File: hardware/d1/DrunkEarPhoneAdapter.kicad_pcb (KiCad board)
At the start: 4 copper layers, 50 x 50 mm, 188 parts, among them J3 SWD, J4 UART, Q1 CSD17577Q3A, Q2 CSD17577Q3A, Q3 DMG1012T-7, SW1 SSSS811101, SW3 DSHP02TSGER, U1 CS43131-CNZR, U10 BLM15PX601SN1D, U11 TPS7A2033PDBVR, U12 TPS7A2018PDBVR, U13 TPS7A2018PDBVR, U14 BLM15PX601SN1D, U15 ESDA25P35-1U1M, U16 ESDA25P35-1U1M, U17 SN74LVC1G32DBVR, U18 TPS22917DBVR, U19 TPS22917DBVR, U2 STM32G0B1VCT6, U20 SN74AVC4T774RSVR, U21 TCA9406DCUR, U3 TS3USB221RSER, U4 TCPP03-M20, U5 TCPP03-M20, U6 ES8327, U7 TPS7A2018PDBVR, U8 TPS7A2033PDBVR, U9 TPS560430XFDBVR, X1 22.5792MHz, X3 24.576MHz

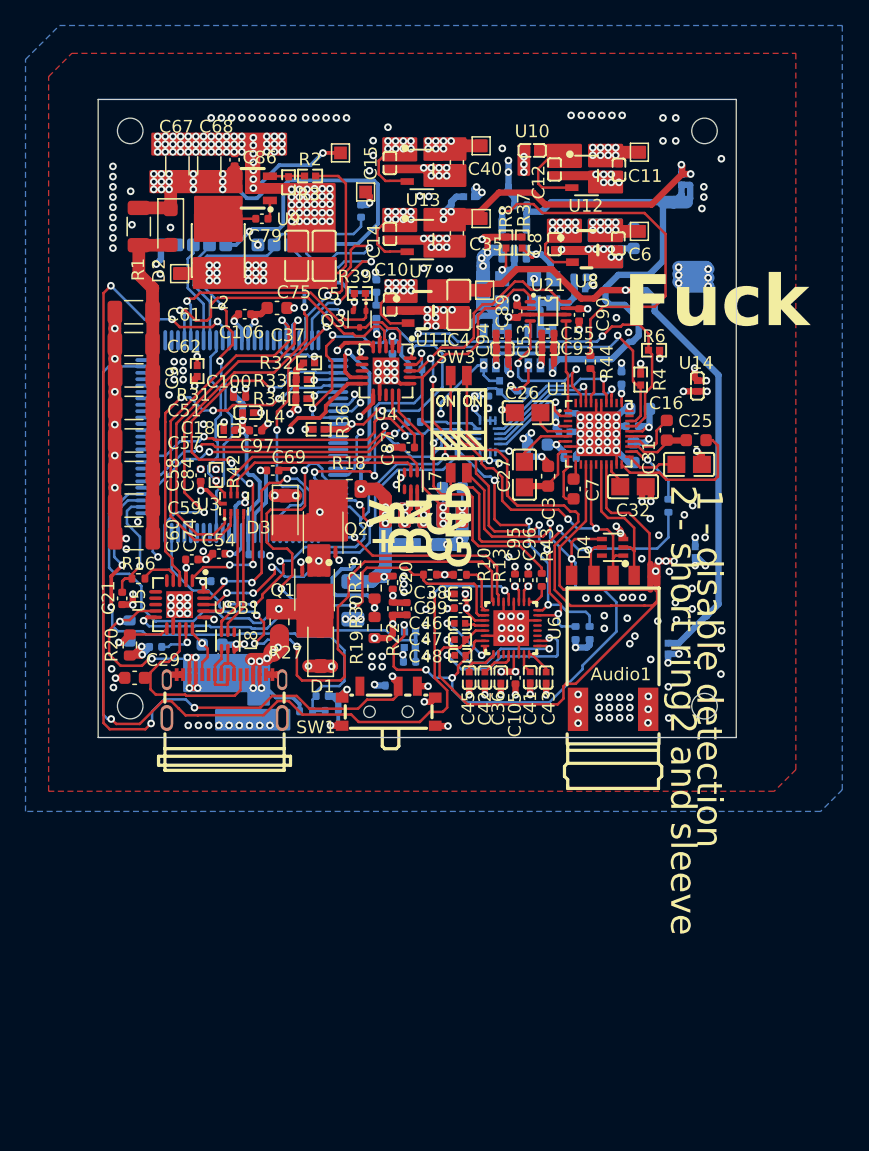
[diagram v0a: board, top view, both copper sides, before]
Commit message: Fixes
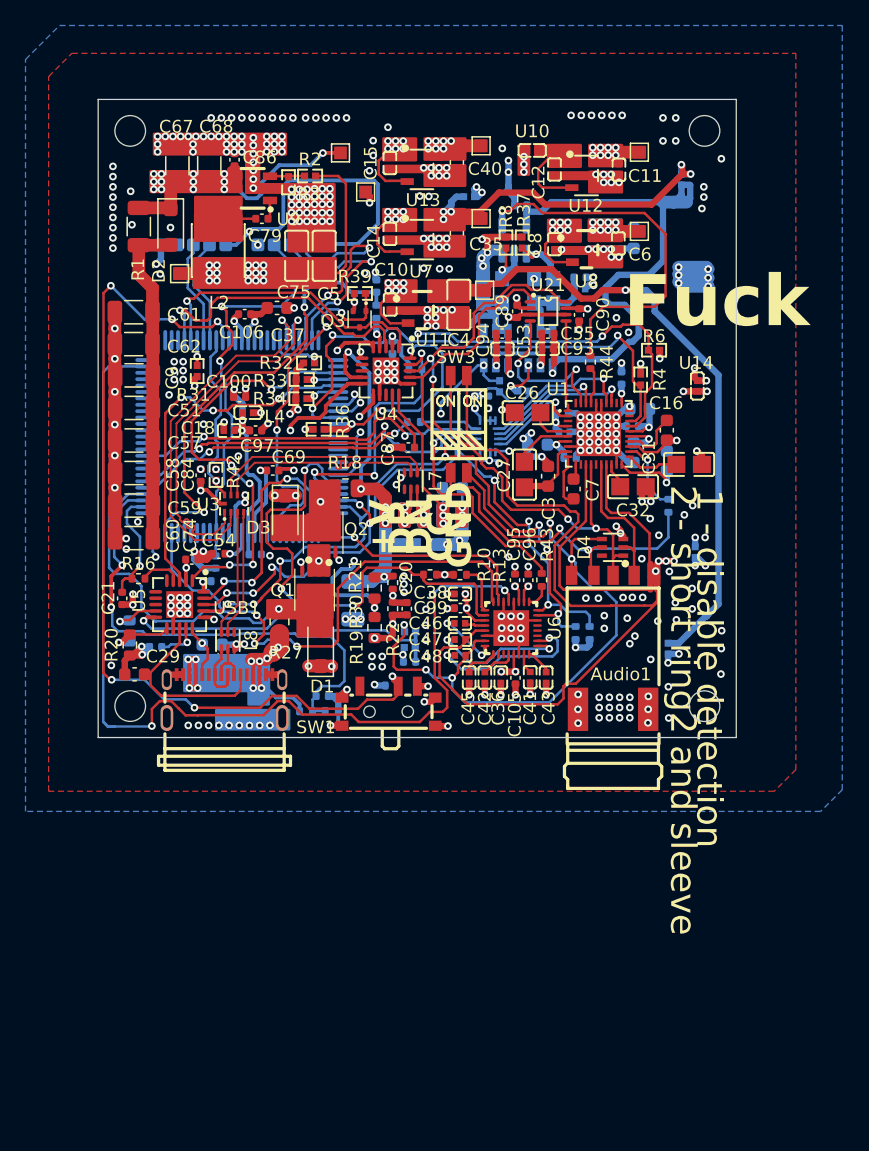
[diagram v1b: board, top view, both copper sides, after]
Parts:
- C25: moved to B.Cu
- moved C56 29.8 mm to (28.5, 54.2), turned to -90 degrees
- moved C25 2.82 mm to (63.9, 46.3), turned to -90 degrees
- moved R18 0.30 mm to (38.7, 48.4)
- moved C29 0.27 mm to (22.2, 63.0)
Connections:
- L7 pad 5: /ucpd/D_P -> /ucpd/D_N
- L7 pad 6: /ucpd/D_N -> /ucpd/D_P
- USBC3 pad 2: /ucpd/D_P -> /ucpd/D_N
- USBC3 pad 3: /ucpd/D_N -> /ucpd/D_P
- USBC4 pad 2: /ucpd/D_P -> /ucpd/D_N
- USBC4 pad 3: /ucpd/D_N -> /ucpd/D_P
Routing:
- net /dac/FLYN_VCP: track 11.7 -> 5.16 mm, vias 0 -> 1
- net /mcu/NRST: track 38.5 -> 32.1 mm
- net /adc/I2S_SD: track 46.8 -> 40.9 mm
- net GND: track 169.3 -> 174.2 mm, vias 398 -> 383
- net /mcu/USB_DIR_SW: track 75.4 -> 70.7 mm
- net /ucpd/USB_CHR_VBUS: track 57.6 -> 61.3 mm, vias 13 -> 12
- net /adc/I2S_CK: track 77.1 -> 79.8 mm
- net PWR_IN: track 88.8 -> 86.7 mm, vias 20 -> 17
- net /adc/GMS1: track 58.4 -> 56.8 mm
- net /mcu/USB_DP: track 28.3 -> 29.8 mm
- net /ucpd/D_N: track 2.23 -> 3.72 mm
- net /ucpd/USB_PHONE_SAFE_DN: track 16.0 -> 17.4 mm
- net +1V8_CP: track 49.3 -> 50.8 mm
- net /dac/JACK_TIP_DETECT: track 29.6 -> 28.4 mm
- net Net-(U20-B3): track 20.8 -> 19.6 mm
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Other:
- outline, holes or cut-outs redrawn
